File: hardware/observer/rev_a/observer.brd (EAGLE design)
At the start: 40.9 x 40.9 mm, 29 parts, among them J1 CON_HEADER_2X05-SMD+SHROUDED, J2 CON_HEADER_2X05-SMD+SHROUDED, J3 TC2030-CC2538-BL-NL, U1 LPS331AP, U2 MPU-9250, U3 SI1147, U4 SI7021, U5 ATUM

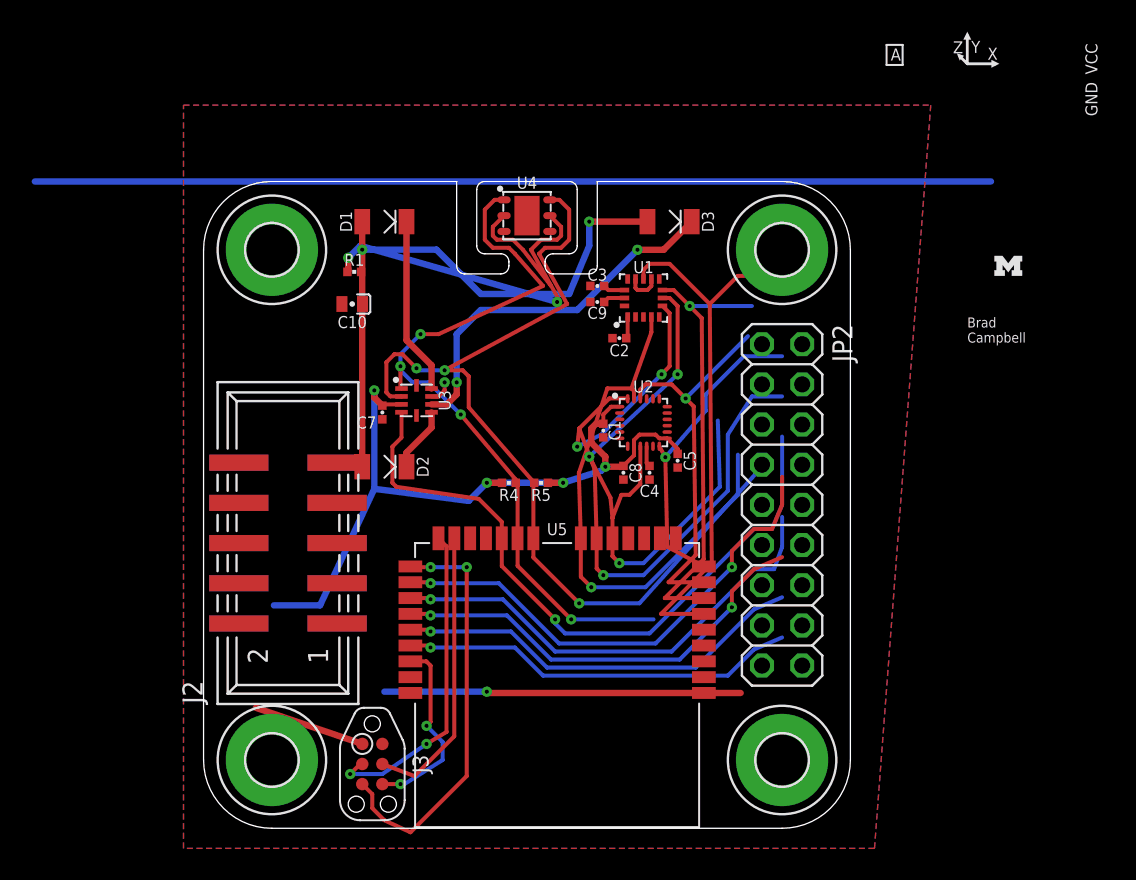
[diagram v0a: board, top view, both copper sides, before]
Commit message: working on sensor board
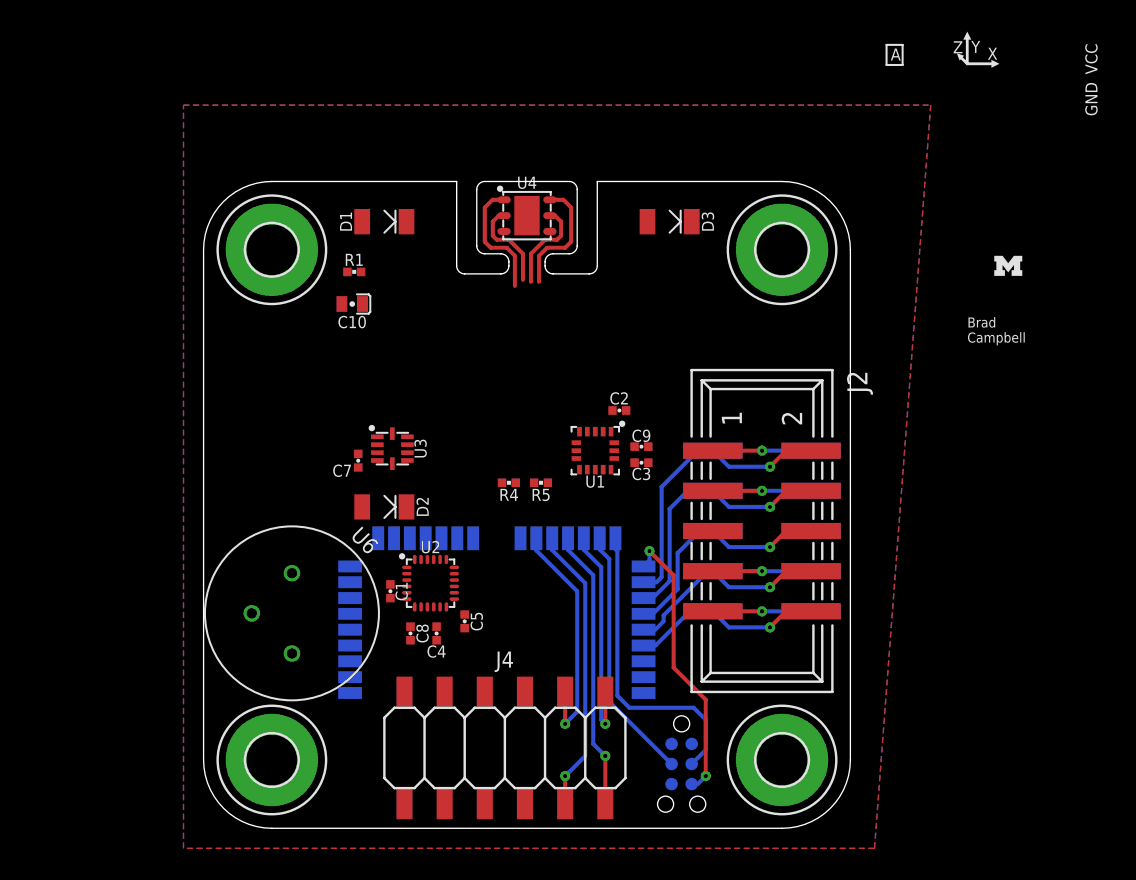
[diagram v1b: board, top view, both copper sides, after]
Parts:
- removed JP2: (no value), pinhead:2X09
- added J4: PINHD-2X6/SMD, headers:2X6/SMD
- added U6: AMN41121, chips:AMN2
- moved J1 30.0 mm to (35.3, 18.8), turned to 270 degrees
- moved J2 30.0 mm to (35.3, 18.8), turned to 270 degrees
- moved J3 19.6 mm to (30.2, 4.06), flipped to the bottom
- moved C1 16.9 mm to (11.8, 15.0)
- moved C4 16.9 mm to (14.7, 12.3)
- moved C5 16.9 mm to (16.5, 13.1)
- moved C8 16.9 mm to (13.1, 12.3)
- moved U2 16.9 mm to (14.4, 15.5)
- moved C3 11.5 mm to (27.7, 23.1), turned to 0 degrees
- moved U1 10.1 mm to (24.8, 23.9), turned to 270 degrees
- moved C9 9.56 mm to (27.7, 24.1), turned to 0 degrees
- moved C2 4.57 mm to (26.3, 26.4), turned to 0 degrees
- moved U5 3.81 mm to (18.5, 18.0), flipped to the bottom
- moved C7 3.41 mm to (9.78, 23.2)
- moved U3 3.41 mm to (11.9, 24.0)
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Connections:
- removed net N$22: JP2.13
- removed net UNUSED: U5.21
- removed net UNUSED2: U5.20
- new net PIR_OUT: U5.7, U6.OUT
- new net UN: U5.6
- net !ACCEL_CS: now also J4.8; no longer JP2.3
- net !BBB_CS: now also U5.28; no longer JP2.12, U5.26
- net !PRESSURE_CS: now also J4.1, J4.11, U5.20; no longer JP2.1, U5.7
- net ACCEL_INT: now also J4.4; no longer JP2.4
- net BBB_INT: now also U5.29; no longer JP2.10, U5.25
- net BBB_MISO: now also U5.26; no longer U5.28
- net BBB_MOSI: now also U5.25; no longer JP2.15, JP2.16, U5.29
- net BBB_SCLK: no longer JP2.14
- net GND: now also U6.GND; no longer JP2.18
- net LIGHT_INT: now also J4.9; no longer JP2.8
- net MISO: now also J4.5; no longer JP2.5
- net MOSI: now also J4.6; no longer JP2.6
- net PRESSURE_INT: now also J4.12, J4.2, U5.21; no longer JP2.2, U5.6
- net SCL: now also J4.3; no longer JP2.9
- net SCLK: now also J4.7; no longer JP2.7
- net SDA: now also J4.10; no longer JP2.11
- net VCC: now also U6.VCC; no longer JP2.17
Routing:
- net VCC: track 105.6 -> 12.1 mm, vias 7 -> 1
- net N$1: track 60.5 -> 0.00 mm
- net SCL: track 59.6 -> 7.76 mm, vias 3 -> 0
- net MOSI: track 44.9 -> 0.00 mm, vias 3 -> 0
- net MISO: track 38.3 -> 0.00 mm, vias 3 -> 0
- net N$8: track 38.2 -> 0.00 mm, vias 2 -> 0
- net SCLK: track 34.4 -> 0.00 mm, vias 1 -> 0
- net LIGHT_INT: track 42.9 -> 18.2 mm
- net !ACCEL_CS: track 24.3 -> 0.00 mm, vias 1 -> 0
- net SDA: track 46.9 -> 22.9 mm, vias 4 -> 1
- net N$7: track 23.5 -> 0.00 mm, vias 2 -> 0
- net PRESSURE_INT: track 34.9 -> 14.3 mm, vias 0 -> 1
- net ACCEL_INT: track 19.8 -> 0.00 mm, vias 1 -> 0
- net BBB_INT: track 31.5 -> 12.3 mm, vias 2 -> 1
- net !BBB_CS: track 29.9 -> 13.4 mm
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
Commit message: basically done with observer
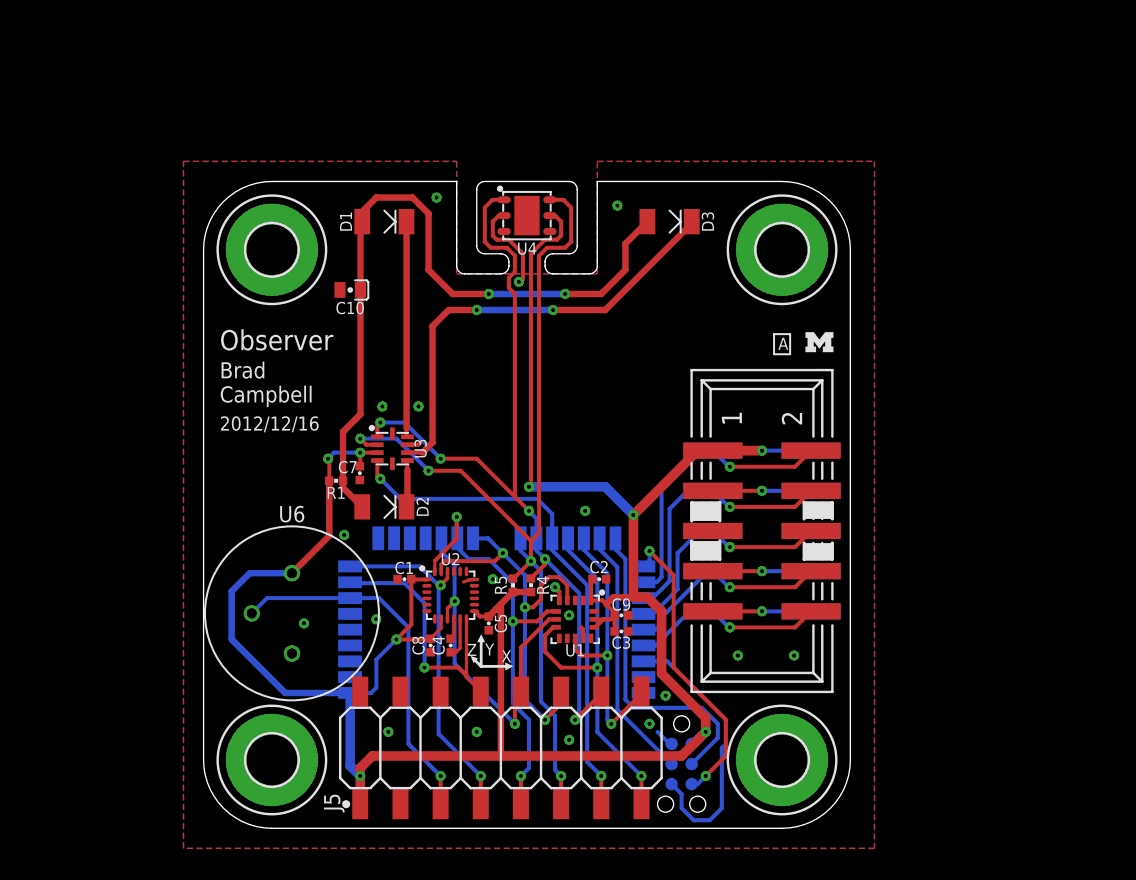
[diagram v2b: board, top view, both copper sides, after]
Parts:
- removed J4: PINHD-2X6/SMD, headers:2X6/SMD
- added J5: PINHD-2X8/SMD, headers:2X8/SMD
- moved R1 13.3 mm to (8.38, 22.0)
- moved LOGO1 12.9 mm to (38.9, 30.7)
- moved C2 10.7 mm to (25.0, 15.7)
- moved C3 10.7 mm to (26.4, 12.4)
- moved U1 10.7 mm to (23.5, 13.2)
- moved C9 10.7 mm to (26.4, 13.5)
- moved R5 6.72 mm to (19.6, 15.4), turned to 270 degrees
- moved R4 6.63 mm to (20.7, 15.4), turned to 270 degrees
- moved C5 1.53 mm to (18.0, 13.0)
- moved C8 1.48 mm to (14.4, 11.6)
- moved U2 1.48 mm to (15.6, 14.7)
- moved C4 1.17 mm to (15.6, 11.6)
- moved C1 1.17 mm to (12.7, 15.7), turned to 180 degrees
- moved C10 0.90 mm to (9.27, 34.0)
- moved C7 0.79 mm to (9.88, 22.5)
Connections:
- new net N$2: J5.3
- new net N$20: J5.4
- new net UNUSED3: J5.6
- net !ACCEL_CS: now also J5.7, U5.9; no longer J4.8, U5.8
- net !PRESSURE_CS: now also J5.15; no longer J4.1, J4.11
- net ACCEL_INT: now also J5.8, U5.8; no longer J4.4, U5.9
- net GND: now also J5.2
- net LIGHT_INT: now also J5.13; no longer J4.9
- net MISO: now also J5.10; no longer J4.5
- net MOSI: now also J5.9; no longer J4.6
- net PIR_OUT: now also J5.5
- net PRESSURE_INT: now also J5.16; no longer J4.12, J4.2
- net SCL: now also J5.11; no longer J4.3
- net SCLK: now also J5.12; no longer J4.7
- net SDA: now also J5.14; no longer J4.10
- net VCC: now also J5.1
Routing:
- net VCC: track 12.1 -> 152.4 mm, vias 1 -> 8
- net SCL: track 7.76 -> 59.9 mm, vias 0 -> 4
- net N$8: track 0.00 -> 45.5 mm, vias 0 -> 2
- net SDA: track 22.9 -> 52.8 mm, vias 1 -> 5
- net N$7: track 0.00 -> 28.4 mm, vias 0 -> 2
- net MOSI: track 0.00 -> 28.0 mm, vias 0 -> 3
- net SCLK: track 0.00 -> 25.9 mm, vias 0 -> 3
- net PIR_OUT: track 0.00 -> 23.1 mm, vias 0 -> 1
- net MISO: track 0.00 -> 22.9 mm, vias 0 -> 2
- net !ACCEL_CS: track 0.00 -> 22.2 mm, vias 0 -> 2
- net !RESET: track 0.00 -> 17.4 mm
- net ACCEL_INT: track 0.00 -> 17.2 mm, vias 0 -> 1
- net LIGHT_INT: track 18.2 -> 32.7 mm, vias 1 -> 2
- net N$4: track 0.00 -> 13.6 mm
- net GND: track 12.0 -> 19.0 mm, vias 1 -> 20
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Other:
- board text added: "2012/12/16"
- board text added: "Observer"
- board text removed: "GND"
- board text removed: "VCC"
